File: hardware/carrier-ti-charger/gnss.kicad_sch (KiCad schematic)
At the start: 28 parts, among them J13 GNSS_ANT, Q14 AO3401A, Q15 2N7002, Q16 2N7002, SW5 ACTIVE_ANT, U16 MAX-M10S-00B, U17 TLV9001IDBVR, U18 TPS7A0233PDBVR

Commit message: Address review findings.
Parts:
- R82: LCSC C17415 -> C727983; MPN 0805W8F100JT5E -> AC0805FR-7W10RL
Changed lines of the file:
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@@
 			)
 		)
-		(property "Description" "Antenna current sense and short limit (UBX-20053088 R8)"
+		(property "Description" "Antenna current sense and short limit, 0.25 W (UBX-20053088 R8)"
 			(at 185.42 132.08 0)
 			(hide yes)
@@
 			)
 		)
-		(property "LCSC" "C17415"
+		(property "LCSC" "C727983"
 			(at 185.42 132.08 0)
 			(hide yes)
@@
 			)
 		)
-		(property "MPN" "0805W8F100JT5E"
+		(property "MPN" "AC0805FR-7W10RL"
 			(at 185.42 132.08 0)
 			(hide yes)

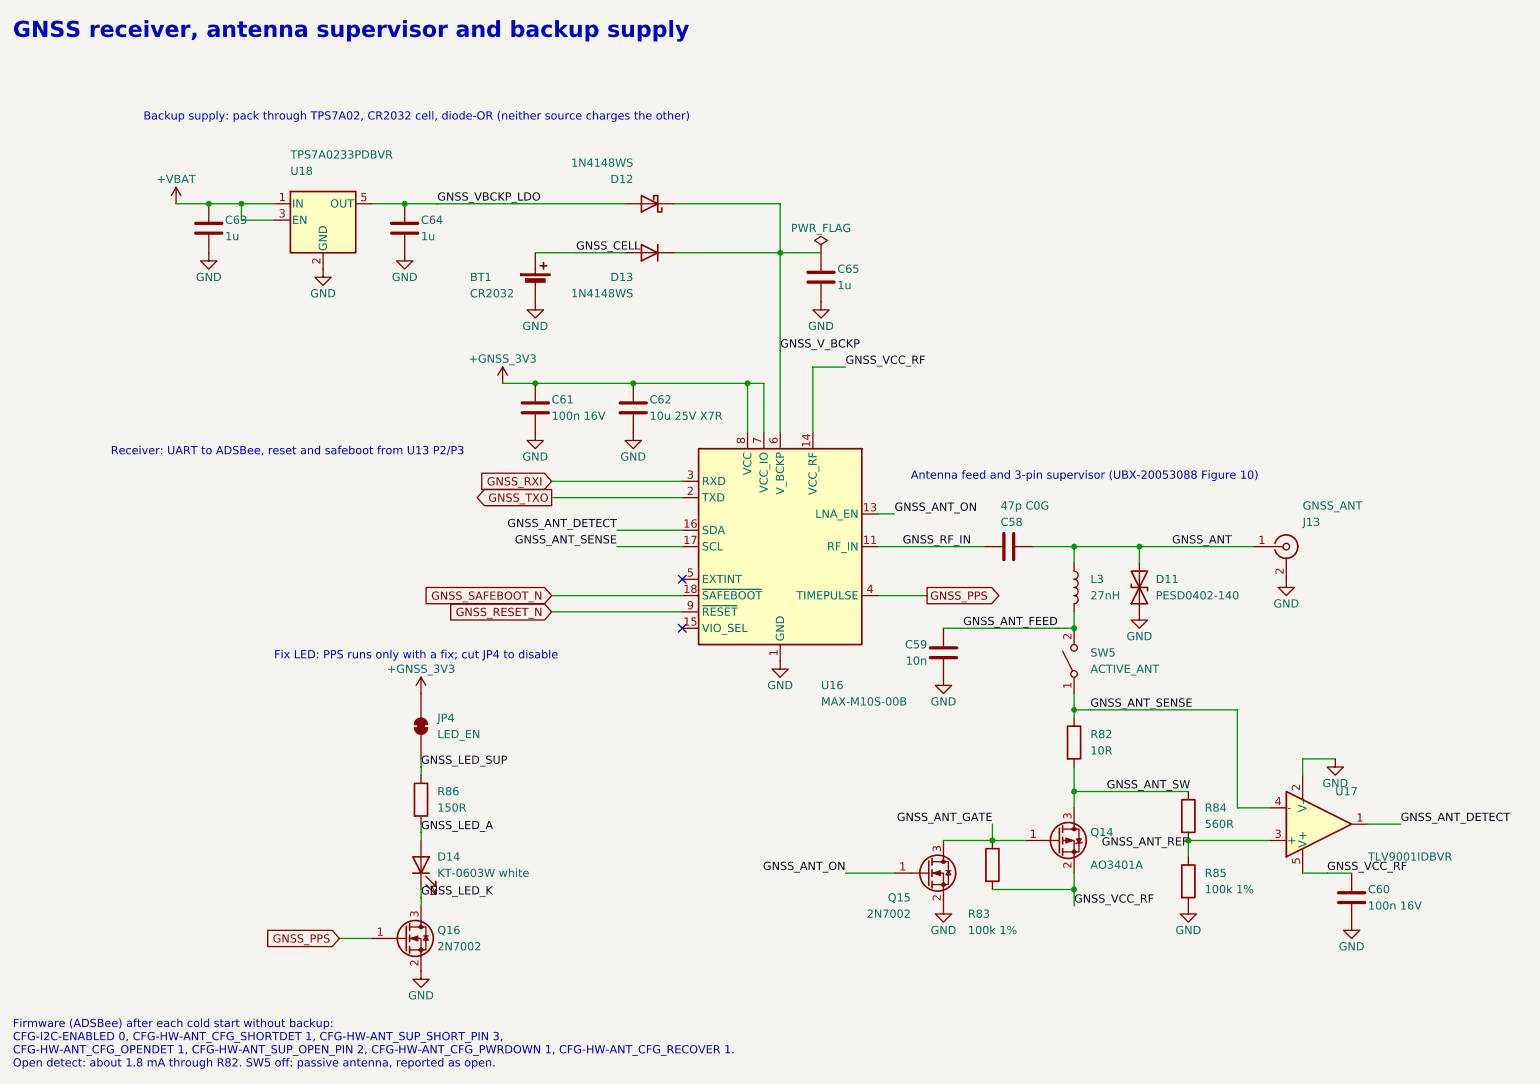
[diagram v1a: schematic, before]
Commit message: Polishing.
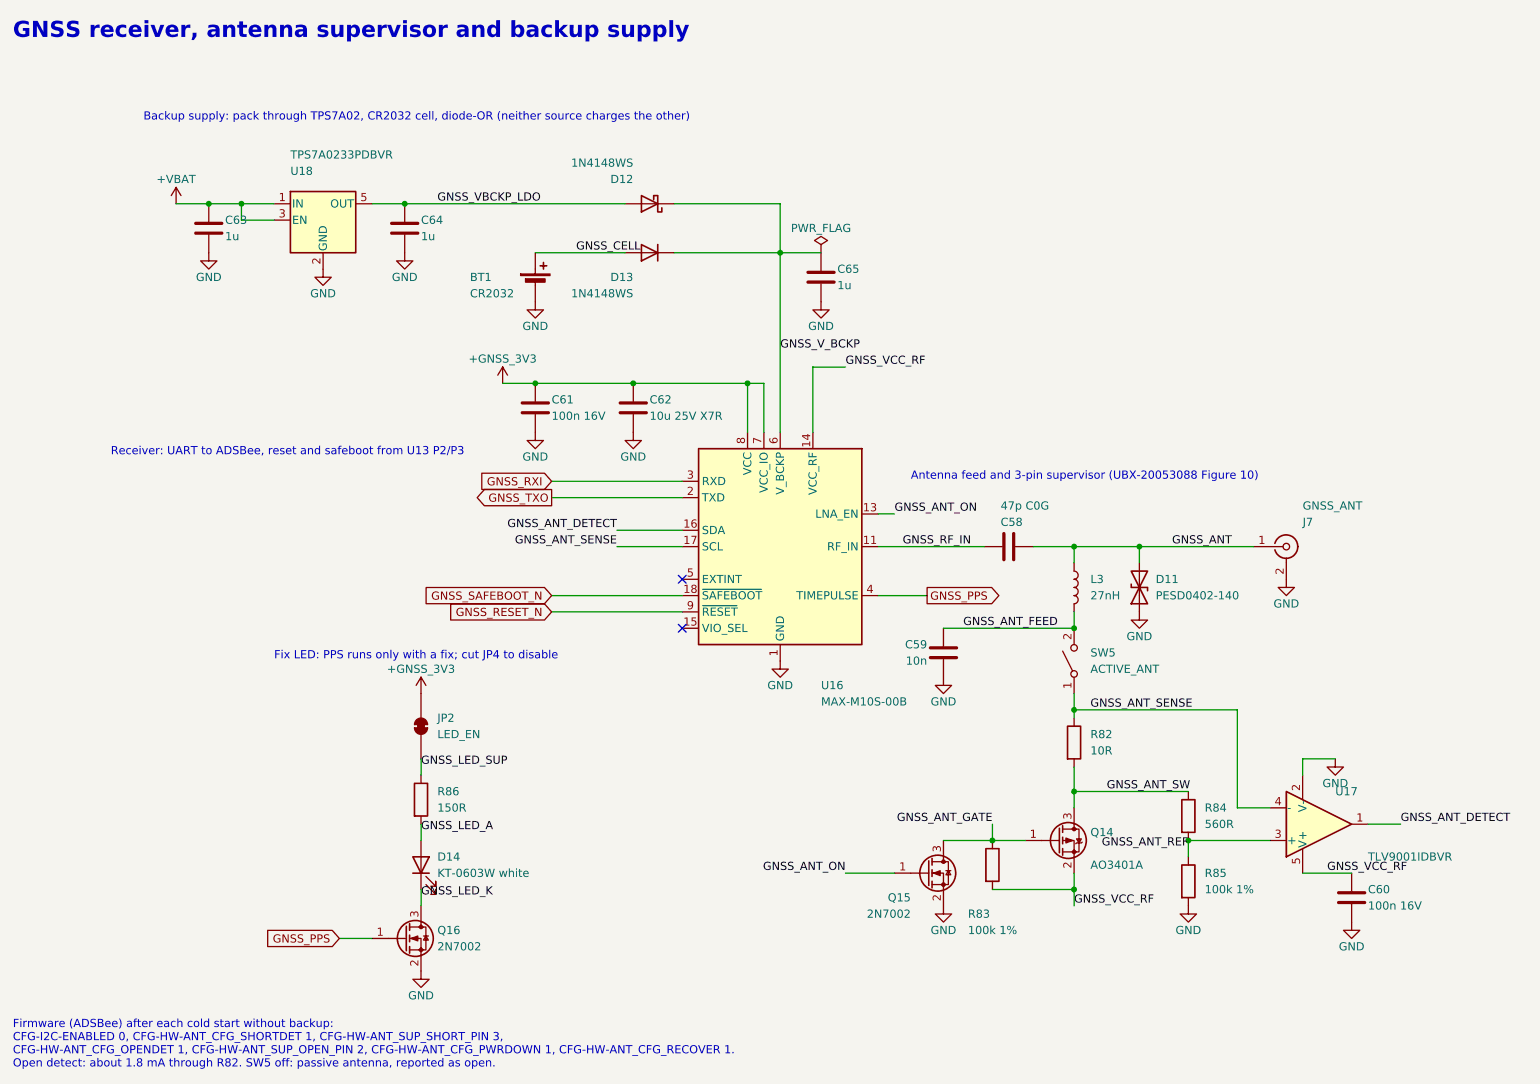
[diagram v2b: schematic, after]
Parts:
- renumbered J13 to J7, JP4 to JP2
